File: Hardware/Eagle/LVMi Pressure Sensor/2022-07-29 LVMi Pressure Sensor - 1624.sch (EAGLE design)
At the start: 26 parts, among them J1 POWER_JACKPJ-102AH, SW1 SWITCH-RA-800BWSP9SM6RE, U1 ATTINY1624-SSU, U2 Sensiron SDP800

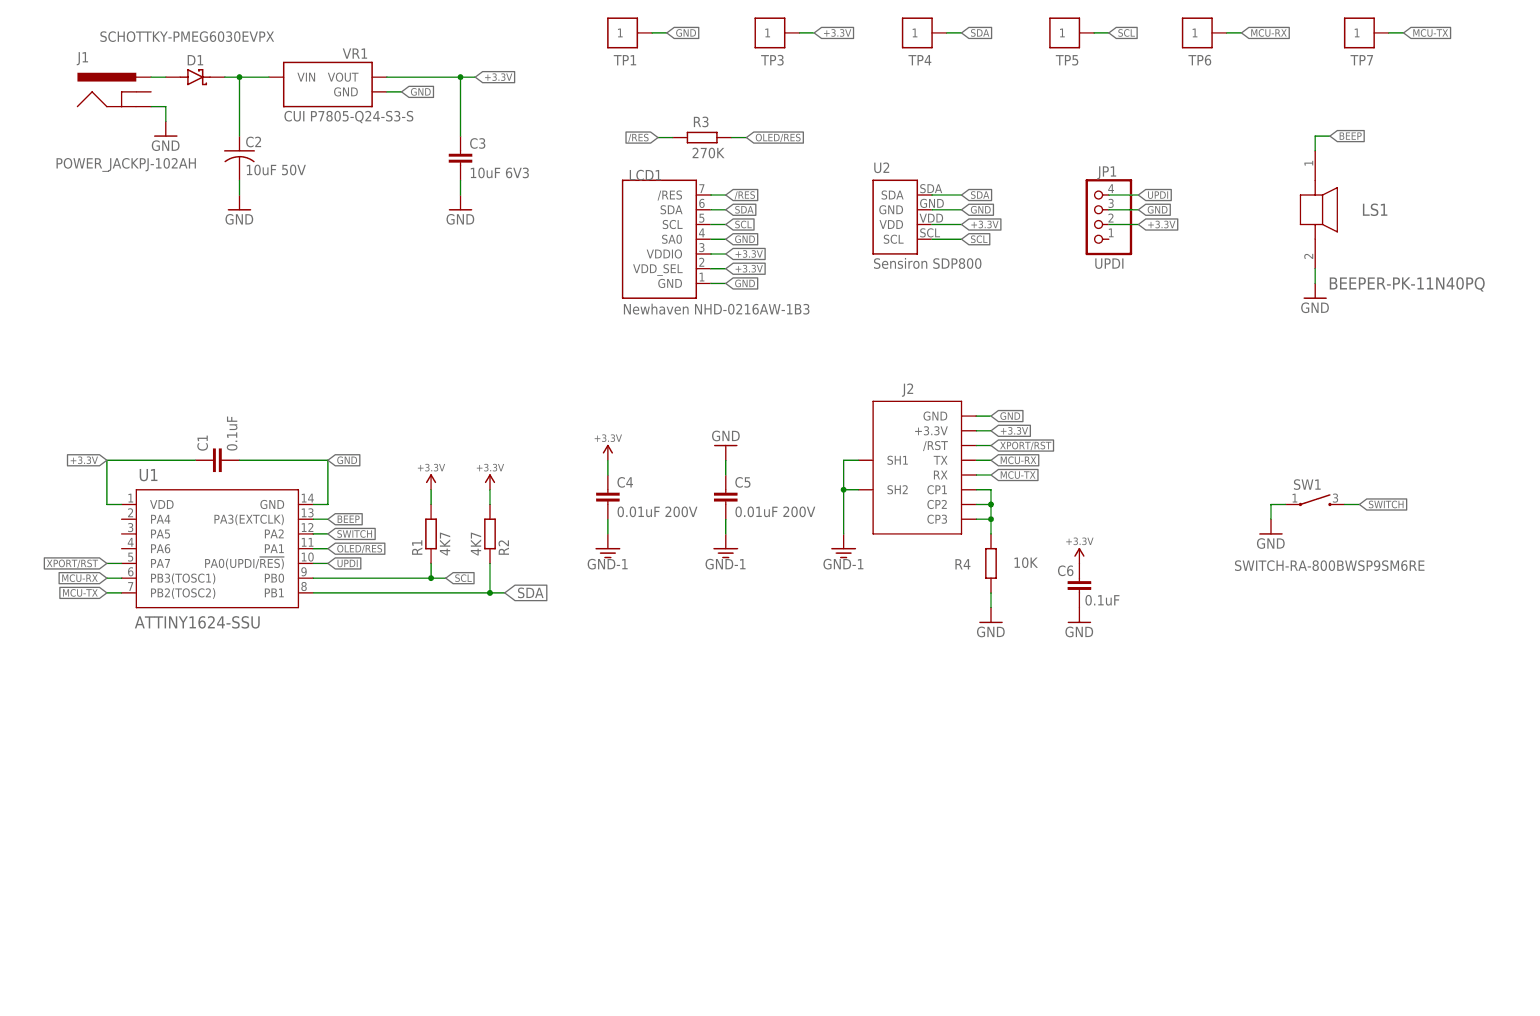
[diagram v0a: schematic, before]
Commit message: WIP
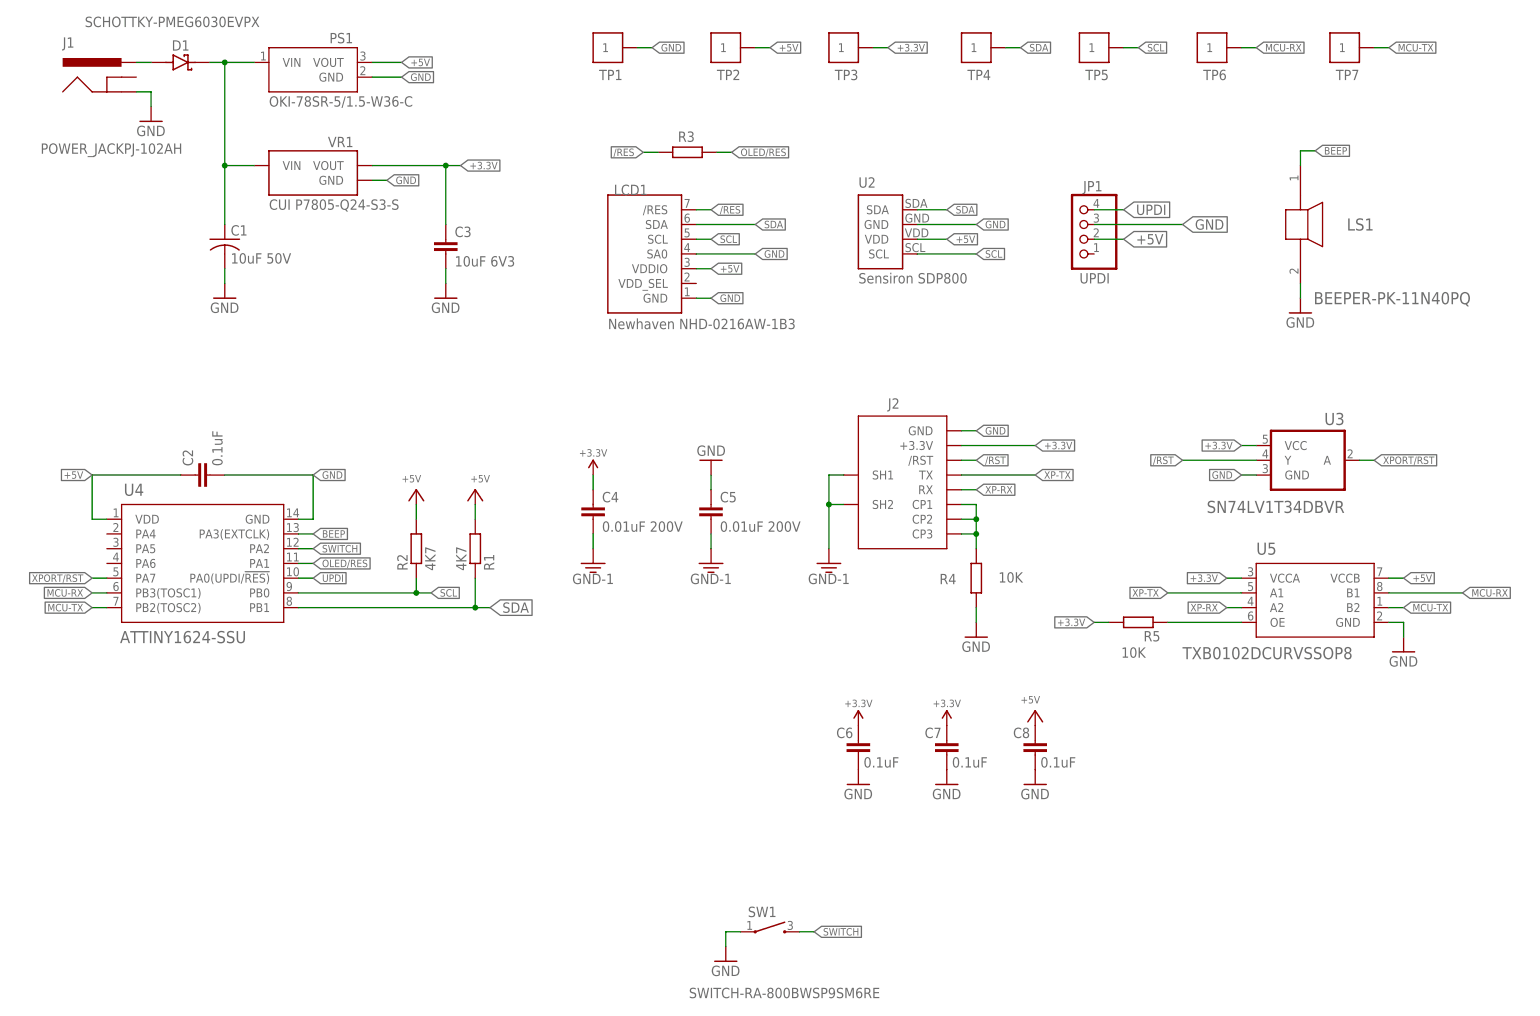
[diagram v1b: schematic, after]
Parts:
- removed U1: ATTINY1624-SSU, AUmlib:ATTINY1624-SSUSOIC150-14_MCH-M
- added C7, C8: 0.1uF, AUmlib:C-EUC0805
- added PS1: OKI-78SR-5/1.5-W36-C, AUmlib:OKI-78SR-5/1.5-W36-C
- added R5: 10K, AUmlib:R-EU_R0805
- added TP2: +5V, AUmlib:TP5000-TESTPOINT-RED
- added U3: SN74LV1T34DBVR, AUmlib:SN74LV1T34DBVR
- added U4: ATTINY1624-SSU, AUmlib:ATTINY1624-SSUSOIC150-14_MCH-M
- added U5: TXB0102DCURVSSOP8, AUmlib:TXB0102DCURVSSOP8
- C1: value 0.1uF -> 10uF 50V; device AUmlib:C-EUC0805 -> AUmlib:C-USC1210
- C2: value 10uF 50V -> 0.1uF; device AUmlib:C-USC1210 -> AUmlib:C-EUC0805
- R3: value 270K -> (none)
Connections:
- new net +5V: C2.1, C8.2, JP1.2, LCD1.VDDIO, PS1.VOUT, R1.2, R2.2, TP2.1, U2.VDD, U4.VDD, U5.VCCB
- new net /RST: J2./RST, U3.Y
- new net OE: R5.1, U5.OE
- new net XP-RX: J2.RX, U5.A2
- new net XP-TX: J2.TX, U5.A1
- net +3.3V: now also C7.2, R5.2, U3.VCC, U5.VCCA; no longer C1.1, JP1.2, LCD1.VDDIO, LCD1.VDD_SEL, R1.2, R2.2, U1.VDD, U2.VDD
- net BEEP: now also U4.PA3(EXTCLK); no longer U1.PA3(EXTCLK)
- net GND: now also C7.1, C8.1, PS1.GND, U3.GND, U4.GND, U5.GND; no longer U1.GND
- net MCU-RX: now also U4.PB3(TOSC1), U5.B1; no longer J2.TX, U1.PB3(TOSC1)
- net MCU-TX: now also U4.PB2(TOSC2), U5.B2; no longer J2.RX, U1.PB2(TOSC2)
- net OLED/RES: now also U4.PA1; no longer U1.PA1
- net SCL: now also R2.1, U4.PB0; no longer R1.1, U1.PB0
- net SDA: now also R1.1, U4.PB1; no longer R2.1, U1.PB1
- net SWITCH: now also U4.PA2; no longer U1.PA2
- net UPDI: now also U4.PA0(UPDI/!RES); no longer U1.PA0(UPDI/!RES)
- net VIN: now also C1.1, PS1.VIN; no longer C2.1
- net XPORT/RST: now also U3.A, U4.PA7; no longer J2./RST, U1.PA7
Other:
- note removed: "Display Switch"
- moved on the sheet: C1, C2, C3, C4, C5, C6, D1, J1, J2, JP1, LCD1, LS1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
